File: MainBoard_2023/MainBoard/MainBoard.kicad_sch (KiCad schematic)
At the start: 45 parts

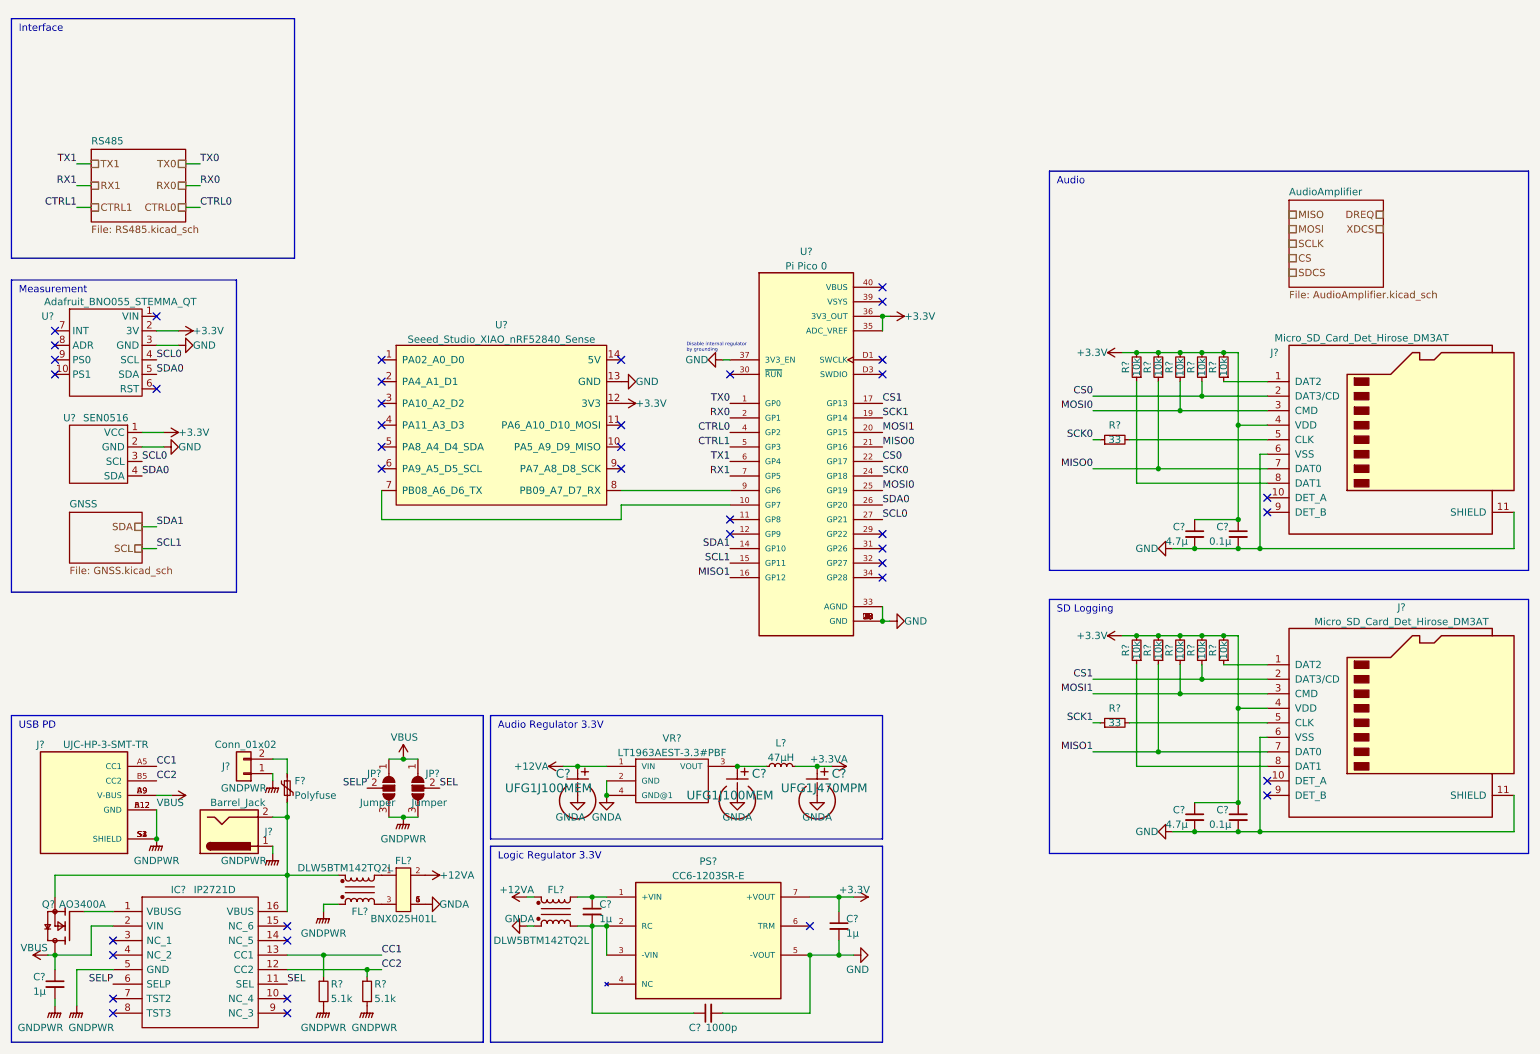
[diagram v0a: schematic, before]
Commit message: メイン基板設計一段落
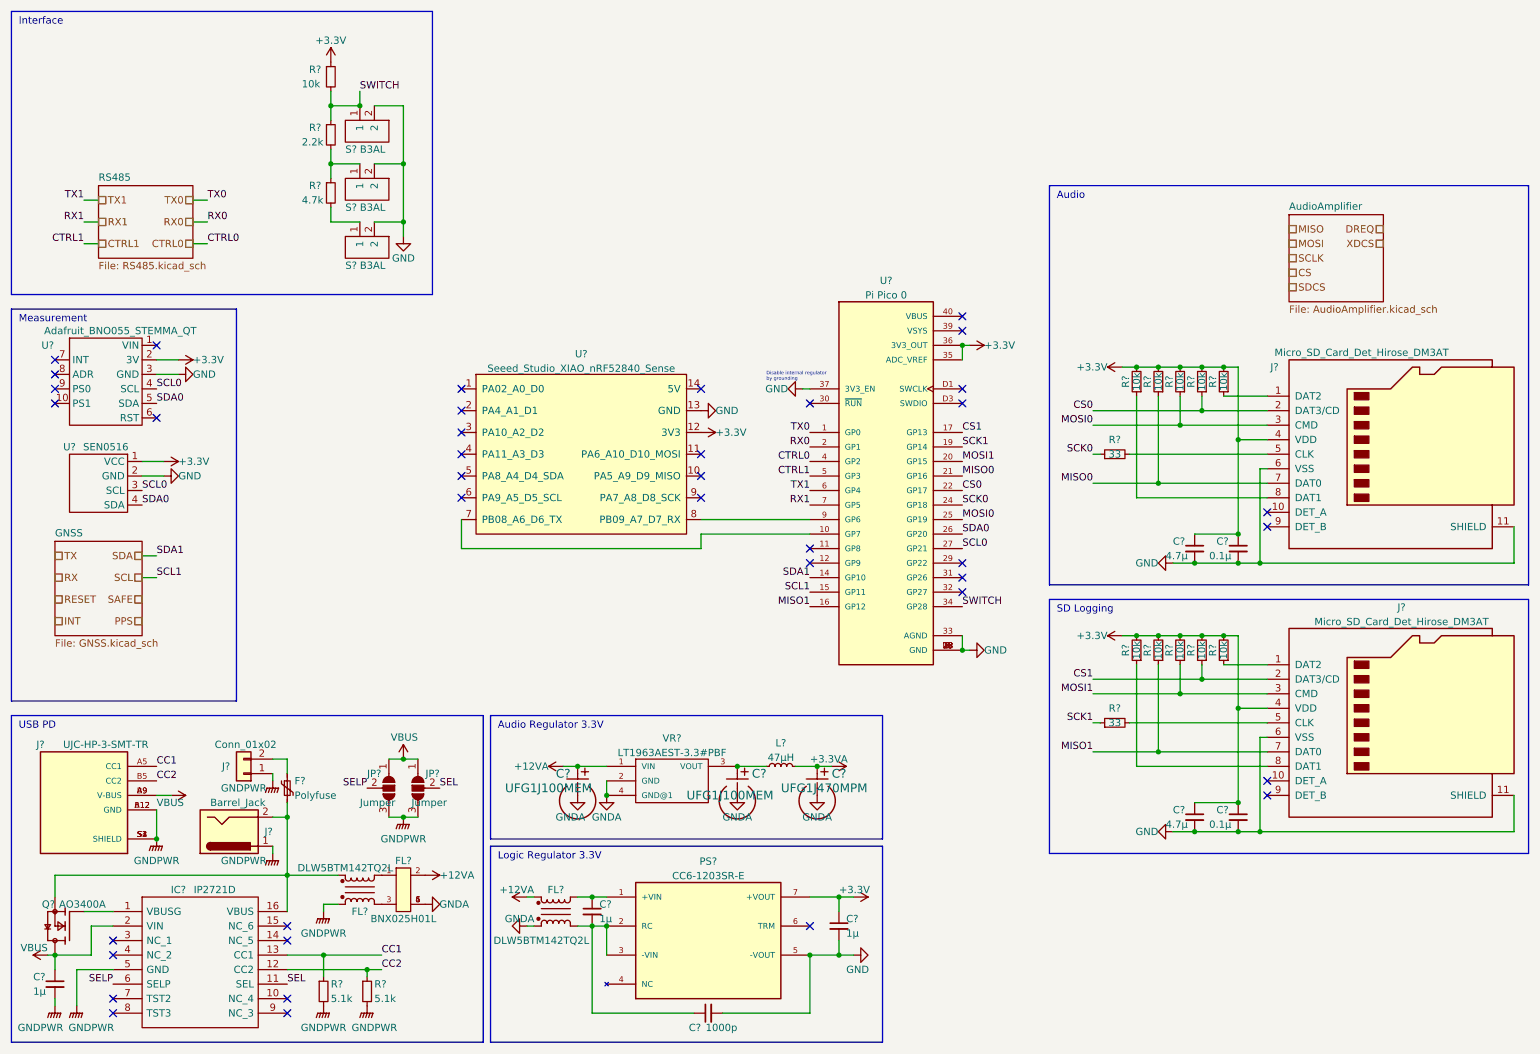
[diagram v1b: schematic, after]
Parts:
- added R?: 4.7k, symbol Device:R_Small
- added R?: 2.2k, symbol Device:R_Small
- added R?: 10k, symbol Device:R_Small
- added S? (x3): B3AL, B3AL1002PMS, symbol B3AL-1002P-MS:B3AL-1002P-MS
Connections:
- net +3.3V: now also R?.1
- net GND: now also S?.2, S?.2, S?.2
- net SWITCH: now reaches U?.34 (GP28)
- net SWITCH: now also R?.1, R?.2, S?.1
- new net: R?.1, R?.2, S?.1
- new net: R?.2, S?.1
- no-connect marks 40 -> 39
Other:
- moved on the sheet: C?, J?, R?, U?
